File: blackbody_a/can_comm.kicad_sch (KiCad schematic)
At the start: 8 parts, among them U2 TCAN337DCNR

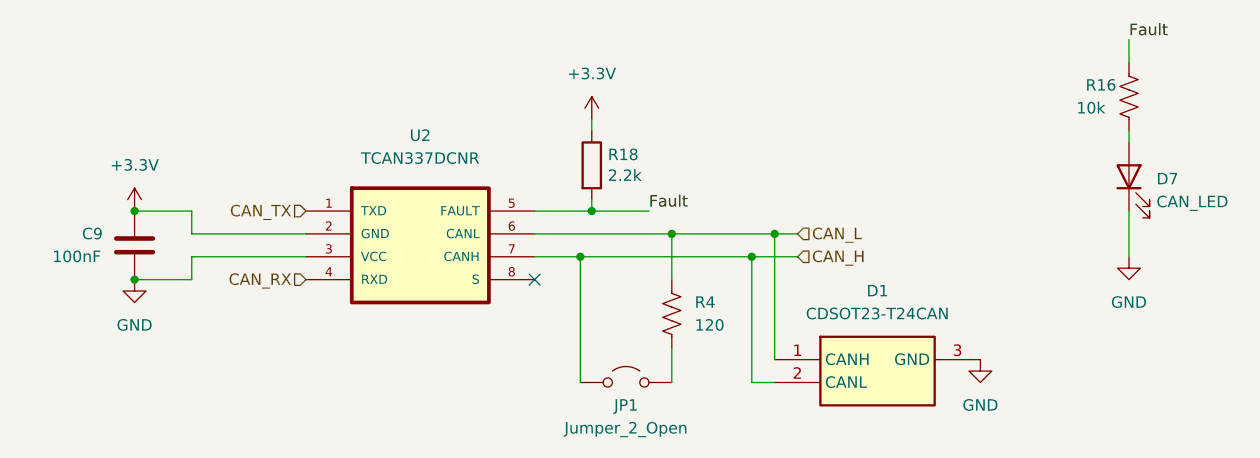
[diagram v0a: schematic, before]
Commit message: layout updates
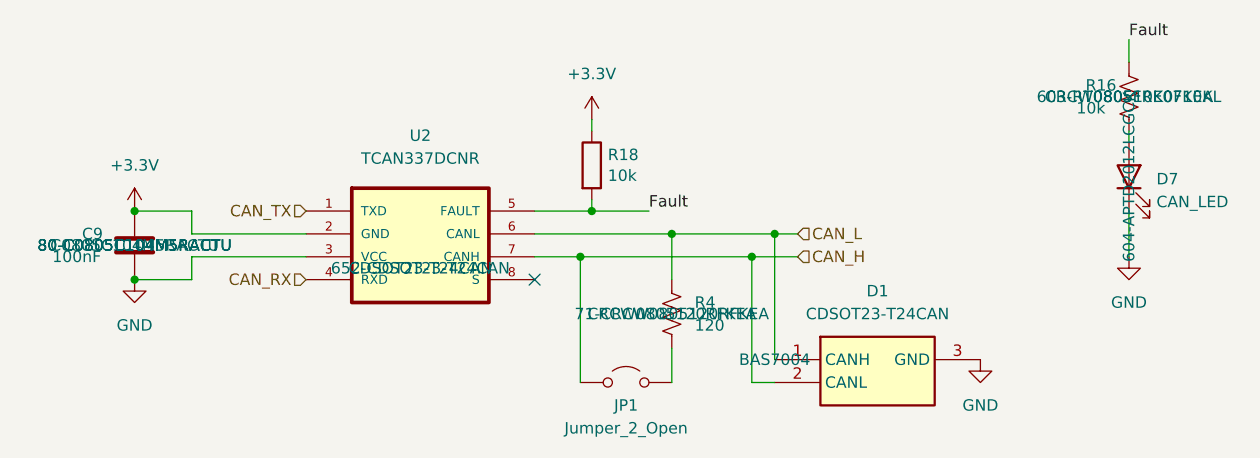
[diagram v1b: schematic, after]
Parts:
- C9: Manufacturer_Part_Number (none) -> 80-C0805C104M5RACTU; Mouser Part Number (none) -> 80-C0805C104M5RACTU; PN (none) -> C0805C104M5RACTU
- D1: Mouser Part Number 652-CDSOT23-T24CAN -> 637-BAS70-04; PN (none) -> BAS7004
- D7: Manufacturer_Part_Number (none) -> 604-APTD2012LCGCK; PN (none) -> APTD2012LCGCK
- R16: Mouser Part Number (none) -> 603-RT0805FRE0710KL; PN (none) -> CRCW080510K0FKEA
- R18: value 2.2k -> 10k; PN (none) -> CRCW080510K0FKEA
- R4: Mouser Part Number (none) -> 71-CRCW0805120RFKEA; PN (none) -> CRCW0805120RFKEA
- U2: Mouser Part Number (none) -> 652-CDSOT23-T24CAN; PN (none) -> CDSOT23-T24CAN
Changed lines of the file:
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@@
+			)
+		)
+		(property "Mouser Part Number" "603-RT0805FRE0710KL"
+			(at 191.77 74.93 0)
+			(effects
+				(font
+					(size 1.27 1.27)
+				)
+			)
+		)
+		(property "PN" "CRCW080510K0FKEA"
+			(at 191.77 74.93 0)
+			(effects
+				(font
+					(size 1.27 1.27)
+				)
 			)
 		)
@@
 			)
 		)
-		(property "PN" ""
+		(property "PN" "APTD2012LCGCK"
 			(at 191.77 83.82 0)
 			(effects
@@
 				)
 				(hide yes)
+			)
+		)
+		(property "Manufacturer_Part_Number" "604-APTD2012LCGCK"
+			(at 191.77 83.82 0)
+			(effects
+				(font
+					(size 1.27 1.27)
+				)
 			)
 		)
@@
 			)
 		)
-		(property "Mouser Part Number" "652-CDSOT23-T24CAN"
+		(property "Mouser Part Number" "637-BAS70-04"
 			(at 171.45 599.06 0)
 			(effects
@@
 				(justify left top)
 				(hide yes)
+			)
+		)
+		(property "PN" "BAS7004"
+			(at 152.4 104.14 0)
+			(effects
+				(font
+					(size 1.27 1.27)
+				)
 			)
 		)
@@
 			)
 		)
+		(property "Mouser Part Number" "71-CRCW0805120RFKEA"
+			(at 140.97 99.06 0)
+			(effects
+				(font
+					(size 1.27 1.27)
+				)
+			)
+		)
+		(property "PN" "CRCW0805120RFKEA"
+			(at 140.97 99.06 0)
+			(effects
+				(font
+					(size 1.27 1.27)
+				)
+			)
+		)
 		(pin "2"
 		)
@@
 			)
 		)
+		(property "Mouser Part Number" "652-CDSOT23-T24CAN"
+			(at 113.03 93.98 0)
+			(effects
+				(font
+					(size 1.27 1.27)
+				)
+			)
+		)
+		(property "PN" "CDSOT23-T24CAN"
+			(at 113.03 93.98 0)
+			(effects
+				(font
+					(size 1.27 1.27)
+				)
+			)
+		)
 		(pin "8"
 		)
@@
 			)
 		)
-		(property "Value" "2.2k"
+		(property "Value" "10k"
 			(at 133.858 83.693 0)
 			(effects
@@
 			)
 		)
-		(property "PN" ""
+		(property "PN" "CRCW080510K0FKEA"
 			(at 132.08 82.55 0)
 			(effects
@@
 			)
 		)
+		(property "Manufacturer_Part_Number" "80-C0805C104M5RACTU"
+			(at 81.28 91.44 0)
+			(effects
+				(font
+					(size 1.27 1.27)
+				)
+			)
+		)
+		(property "Mouser Part Number" "80-C0805C104M5RACTU"
+			(at 81.28 91.44 0)
+			(effects
+				(font
+					(size 1.27 1.27)
+				)
+			)
+		)
+		(property "PN" "C0805C104M5RACTU"
+			(at 81.28 91.44 0)
+			(effects
+				(font
+					(size 1.27 1.27)
+				)
+			)
+		)
